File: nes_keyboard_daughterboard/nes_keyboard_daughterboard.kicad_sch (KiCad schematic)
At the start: 17 parts, among them J1 USB_C_Receptacle_USB2.0_16P, J2 Conn_01x02_Pin, J3 USB_C_Receptacle_USB2.0_16P, U1 NCP1117-3.3_SOT223, U2 USBLC6-2P6

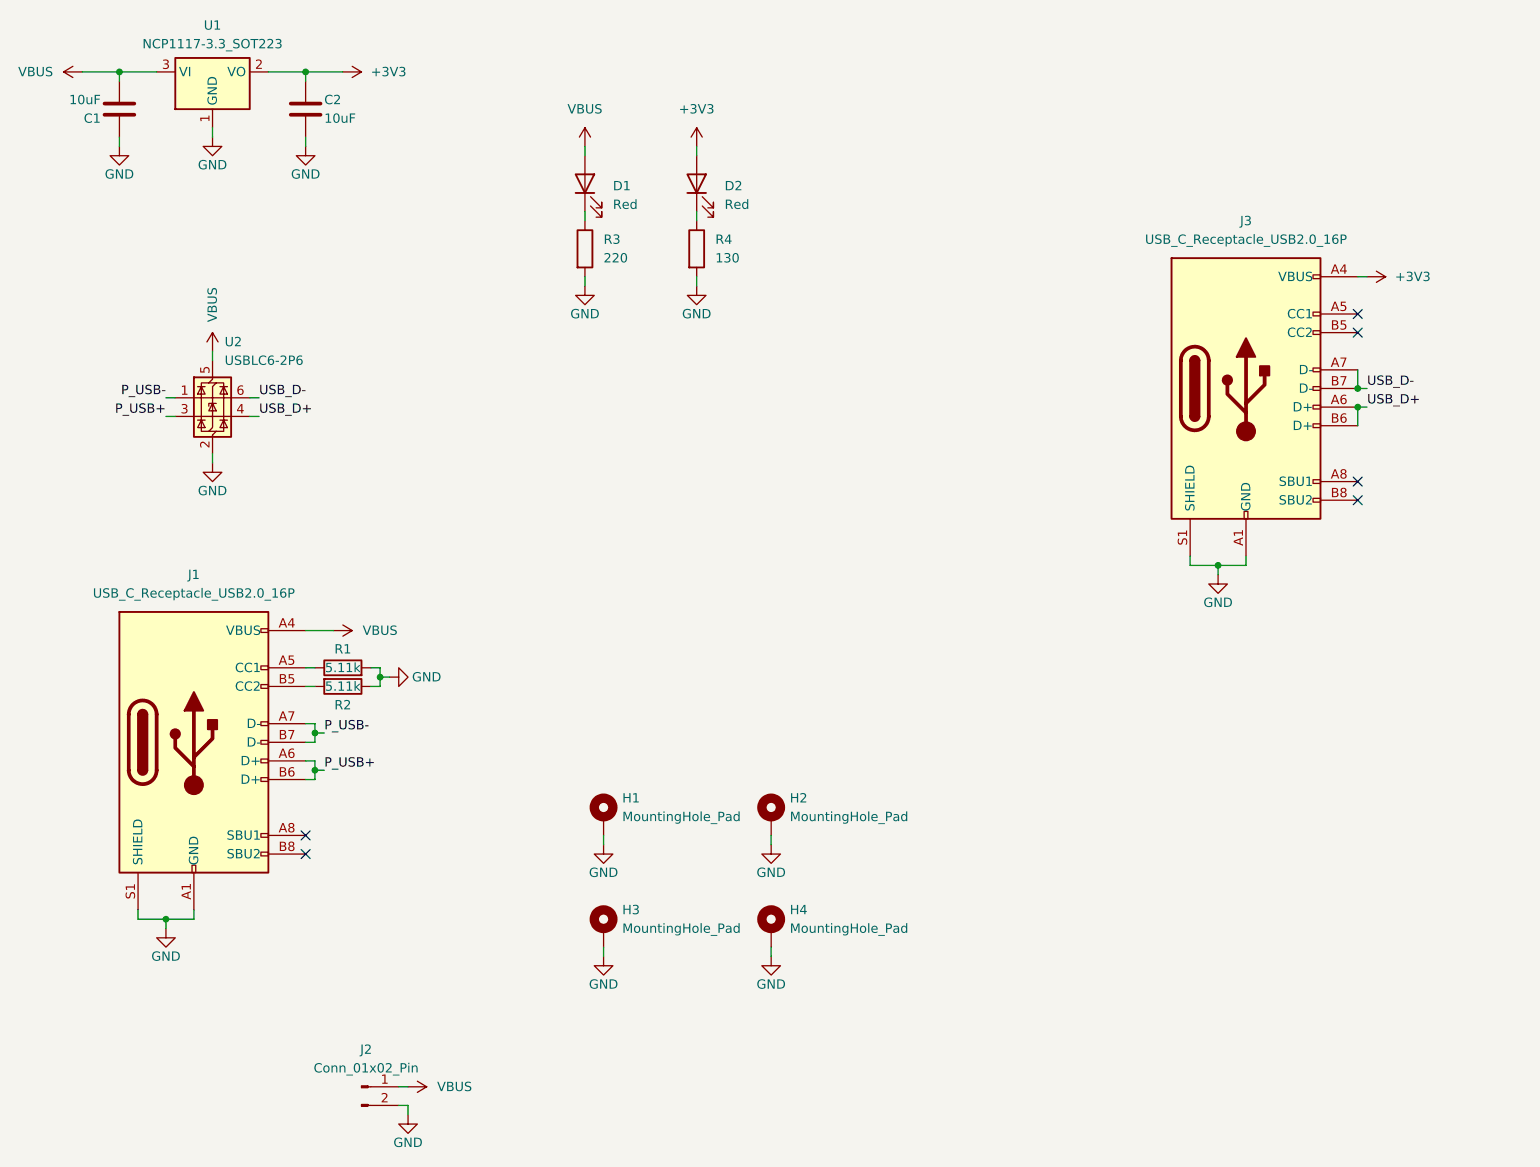
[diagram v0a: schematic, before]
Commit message: Finished V0.1
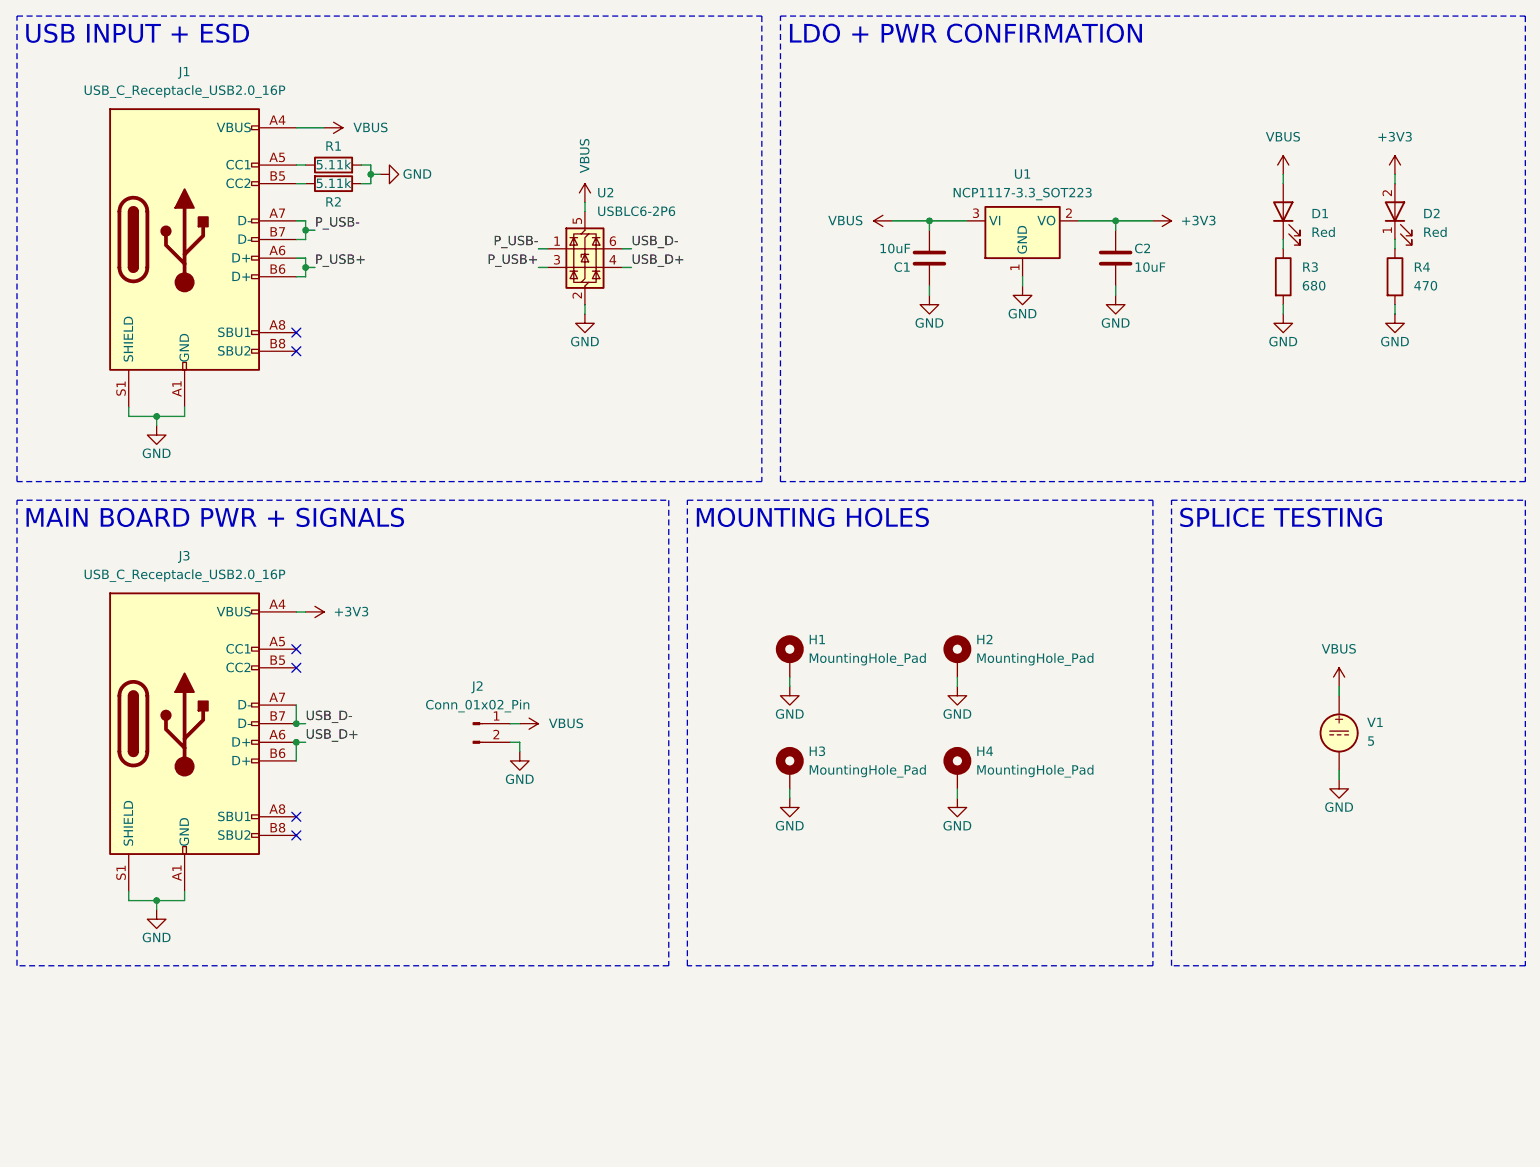
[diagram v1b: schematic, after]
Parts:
- added V1: 5, symbol Simulation_SPICE:VDC
- R3: value 220 -> 680
- R4: value 130 -> 470
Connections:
- net GND: now also V1.2
- net VBUS: now also V1.1
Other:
- moved on the sheet: C1, C2, D1, H1, H2, H3, H4, J1, J2, J3, R1, R2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

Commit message: PCB Modifications (all) - V0.2
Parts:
- C1, C2: footprint Capacitor_SMD:C_0603_1608Metric_Pad1.08x0.95mm_HandSolder -> Capacitor_SMD:C_0805_2012Metric_Pad1.18x1.45mm_HandSolder; LCSC (none) -> C95841
- D1, D2: LCSC (none) -> C19171390
- J1: LCSC (none) -> C7095263
- J2: footprint Connector_Hirose:Hirose_DF13-02P-1.25DSA_1x02_P1.25mm_Vertical -> Connector_JST:JST_PH_S2B-PH-K_1x02_P2.00mm_Horizontal; LCSC (none) -> C17264620
- J3: LCSC (none) -> C3020560
- R1, R2: LCSC (none) -> C112314
- R3: LCSC (none) -> C112310
- R4: LCSC (none) -> C114433
- U1: LCSC (none) -> C26537
- U2: LCSC (none) -> C15999
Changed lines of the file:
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@@
 			)
 		)
+		(property "LCSC" ""
+			(at 130.81 128.27 0)
+			(hide yes)
+			(show_name no)
+			(do_not_autoplace no)
+			(effects
+				(font
+					(size 1.27 1.27)
+				)
+			)
+		)
 		(pin "1"
 		)
@@
 			)
 		)
-		(property "Footprint" "Connector_Hirose:Hirose_DF13-02P-1.25DSA_1x02_P1.25mm_Vertical"
+		(property "Footprint" "Connector_JST:JST_PH_S2B-PH-K_1x02_P2.00mm_Horizontal"
 			(at 87.63 121.92 0)
 			(hide yes)
@@
 			)
 		)
+		(property "LCSC" "C17264620"
+			(at 87.63 121.92 0)
+			(hide yes)
+			(show_name no)
+			(do_not_autoplace no)
+			(effects
+				(font
+					(size 1.27 1.27)
+				)
+			)
+		)
 		(pin "1"
 		)
@@
 			)
 		)
+		(property "LCSC" "C19171390"
+			(at 213.36 52.07 90)
+			(hide yes)
+			(show_name no)
+			(do_not_autoplace no)
+			(effects
+				(font
+					(size 1.27 1.27)
+				)
+			)
+		)
 		(pin "1"
 		)
@@
 			)
 		)
+		(property "LCSC" ""
+			(at 130.81 113.03 0)
+			(hide yes)
+			(show_name no)
+			(do_not_autoplace no)
+			(effects
+				(font
+					(size 1.27 1.27)
+				)
+			)
+		)
 		(pin "1"
 		)
@@
 			)
 		)
-		(property "Footprint" "Capacitor_SMD:C_0603_1608Metric_Pad1.08x0.95mm_HandSolder"
+		(property "Footprint" "Capacitor_SMD:C_0805_2012Metric_Pad1.18x1.45mm_HandSolder"
 			(at 148.8948 54.61 0)
 			(hide yes)
@@
 			)
 		)
+		(property "LCSC" "C95841"
+			(at 149.86 58.42 0)
+			(hide yes)
+			(show_name no)
+			(do_not_autoplace no)
+			(effects
+				(font
+					(size 1.27 1.27)
+				)
+			)
+		)
 		(pin "1"
 		)
@@
 			)
 		)
+		(property "LCSC" "C3020560"
+			(at 48.26 121.92 0)
+			(hide yes)
+			(show_name no)
+			(do_not_autoplace no)
+			(effects
+				(font
+					(size 1.27 1.27)
+				)
+			)
+		)
 		(pin "B1"
 		)
@@
 			)
 		)
+		(property "LCSC" "C112314"
+			(at 68.58 48.26 90)
+			(hide yes)
+			(show_name no)
+			(do_not_autoplace no)
+			(effects
+				(font
+					(size 1.27 1.27)
+				)
+			)
+		)
 		(pin "1"
 		)
@@
 			)
 		)
+		(property "LCSC" "C19171390"
+			(at 198.12 52.07 90)
+			(hide yes)
+			(show_name no)
+			(do_not_autoplace no)
+			(effects
+				(font
+					(size 1.27 1.27)
+				)
+			)
+		)
 		(pin "1"
 		)
@@
 			)
 		)
+		(property "LCSC" "C26537"
+			(at 162.56 53.34 0)
+			(hide yes)
+			(show_name no)
+			(do_not_autoplace no)
+			(effects
+				(font
+					(size 1.27 1.27)
+				)
+			)
+		)
 		(pin "2"
 		)
@@
 			)
 		)
+		(property "LCSC" "C7095263"
+			(at 48.26 55.88 0)
+			(hide yes)
+			(show_name no)
+			(do_not_autoplace no)
+			(effects
+				(font
+					(size 1.27 1.27)
+				)
+			)
+		)
 		(pin "A4"
 		)
@@
 			)
 		)
+		(property "LCSC" "C112314"
+			(at 68.58 45.72 90)
+			(hide yes)
+			(show_name no)
+			(do_not_autoplace no)
+			(effects
+				(font
+					(size 1.27 1.27)
+				)
+			)
+		)
 		(pin "1"
 		)
@@
 			)
 		)
+		(property "LCSC" ""
+			(at 153.67 128.27 0)
+			(hide yes)
+			(show_name no)
+			(do_not_autoplace no)
+			(effects
+				(font
+					(size 1.27 1.27)
+				)
+			)
+		)
 		(pin "1"
 		)
@@
 			)
 		)
+		(property "LCSC" "C15999"
+			(at 102.87 57.15 0)
+			(hide yes)
+			(show_name no)
+			(do_not_autoplace no)
+			(effects
+				(font
+					(size 1.27 1.27)
+				)
+			)
+		)
 		(pin "1"
 		)
@@
 			)
 		)
+		(property "LCSC" ""
+			(at 205.74 123.19 0)
+			(hide yes)
+			(show_name no)
+			(do_not_autoplace no)
+			(effects
+				(font
+					(size 1.27 1.27)
+				)
+			)
+		)
 		(pin "2"
 		)
@@
 			)
 		)
+		(property "LCSC" "C112310"
+			(at 198.12 60.96 0)
+			(hide yes)
+			(show_name no)
+			(do_not_autoplace no)
+			(effects
+				(font
+					(size 1.27 1.27)
+				)
+			)
+		)
 		(pin "2"
 		)
@@
 			)
 		)
+		(property "LCSC" ""
+			(at 153.67 113.03 0)
+			(hide yes)
+			(show_name no)
+			(do_not_autoplace no)
+			(effects
+				(font
+					(size 1.27 1.27)
+				)
+			)
+		)
 		(pin "1"
 		)
@@
 			)
 		)
-		(property "Footprint" "Capacitor_SMD:C_0603_1608Metric_Pad1.08x0.95mm_HandSolder"
+		(property "Footprint" "Capacitor_SMD:C_0805_2012Metric_Pad1.18x1.45mm_HandSolder"
 			(at 174.2948 54.61 0)
 			(hide yes)
@@
 			)
 		)
+		(property "LCSC" "C95841"
+			(at 175.26 58.42 0)
+			(hide yes)
+			(show_name no)
+			(do_not_autoplace no)
+			(effects
+				(font
+					(size 1.27 1.27)
+				)
+			)
+		)
 		(pin "1"
 		)
@@
 			(at 213.36 60.96 0)
 			(hide yes)
+			(show_name no)
+			(do_not_autoplace no)
+			(effects
+				(font
+					(size 1.27 1.27)
+				)
+			)
+		)
+		(property "LCSC" "C114433"
+			(at 213.36 60.96 0)
+			(hide yes)
